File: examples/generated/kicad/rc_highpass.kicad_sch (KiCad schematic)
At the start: 3 parts

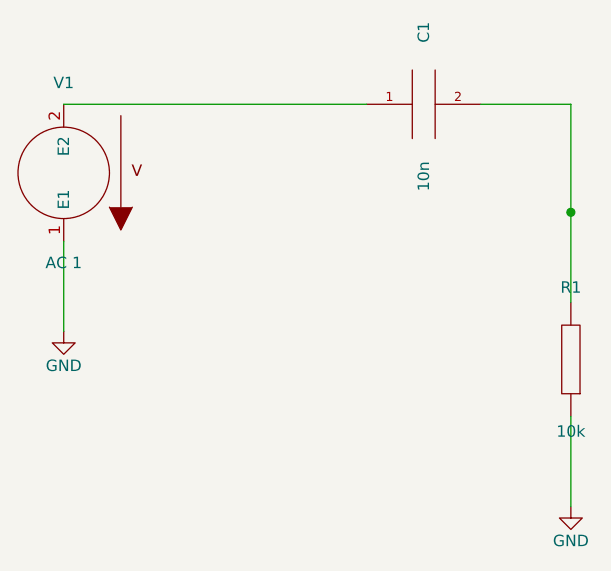
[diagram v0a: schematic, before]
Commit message: Attempt to fix more terminal issues.
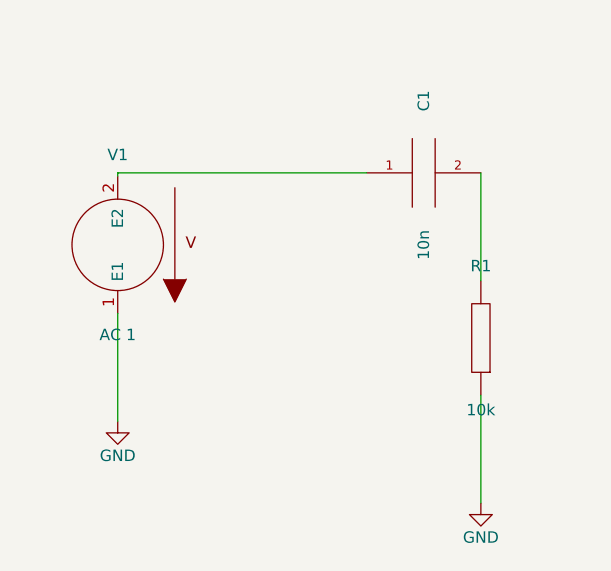
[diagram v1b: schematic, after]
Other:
- moved on the sheet: C1, R1, V1
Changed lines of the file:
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@@
     (comment 1 "Generated by mixedsig2cad")
   )
-  (symbol (lib_id "VSOURCE") (at 50.00 78.00 180) (unit 1)
+  (symbol (lib_id "VSOURCE") (at 56.00 86.00 180) (unit 1)
     (in_bom yes) (on_board yes)
-    (property "Reference" "V1" (at 50.0 68.0 0)
+    (property "Reference" "V1" (at 56.0 76.0 0)
       (effects (font (size 1.27 1.27)))
     )
-    (property "Value" "AC 1" (at 50.0 88.0 0)
+    (property "Value" "AC 1" (at 56.0 96.0 0)
       (effects (font (size 1.27 1.27)))
     )
@@
     )
   )
-  (symbol (lib_id "CAP") (at 90.00 70.38 90) (unit 1)
+  (symbol (lib_id "GND") (at 56.00 105.62 0) (unit 1)
     (in_bom yes) (on_board yes)
-    (property "Reference" "C1" (at 90.0 62.379999999999995 0)
-      (effects (font (size 1.27 1.27)))
+    (property "Reference" "#PWR0001" (at 56.0 101.81 0)
+      (effects (font (size 1.27 1.27)) hide)
     )
-    (property "Value" "10n" (at 90.0 78.38 0)
+    (property "Value" "GND" (at 56.0 109.43 0)
       (effects (font (size 1.27 1.27)))
     )
@@
     )
   )
-  (symbol (lib_id "R") (at 106.35 98.73 180) (unit 1)
+  (symbol (lib_id "CAP") (at 90.00 78.00 90) (unit 1)
     (in_bom yes) (on_board yes)
-    (property "Reference" "R1" (at 106.35 90.73 0)
+    (property "Reference" "C1" (at 90.0 70.0 0)
       (effects (font (size 1.27 1.27)))
     )
-    (property "Value" "10k" (at 106.35 106.73 0)
+    (property "Value" "10n" (at 90.0 86.0 0)
       (effects (font (size 1.27 1.27)))
     )
@@
     )
   )
-  (symbol (lib_id "GND") (at 50.00 95.62 0) (unit 1)
+  (symbol (lib_id "R") (at 96.35 96.35 180) (unit 1)
     (in_bom yes) (on_board yes)
-    (property "Reference" "#PWR0001" (at 50.0 91.81 0)
-      (effects (font (size 1.27 1.27)) hide)
+    (property "Reference" "R1" (at 96.35 88.35 0)
+      (effects (font (size 1.27 1.27)))
     )
-    (property "Value" "GND" (at 50.0 99.43 0)
+    (property "Value" "10k" (at 96.35 104.35 0)
       (effects (font (size 1.27 1.27)))
     )
@@
     )
   )
-  (symbol (lib_id "GND") (at 106.35 115.08 0) (unit 1)
+  (symbol (lib_id "GND") (at 96.35 114.70 0) (unit 1)
     (in_bom yes) (on_board yes)
-    (property "Reference" "#PWR0002" (at 106.35 111.27 0)
+    (property "Reference" "#PWR0002" (at 96.35 110.89 0)
       (effects (font (size 1.27 1.27)) hide)
     )
-    (property "Value" "GND" (at 106.35 118.89 0)
+    (property "Value" "GND" (at 96.35 118.51 0)
       (effects (font (size 1.27 1.27)))
     )
@@
     )
   )
-  (wire (pts (xy 50.00 70.38) (xy 83.65 70.38))
+  (wire (pts (xy 96.35 102.70) (xy 96.35 114.70))
     (stroke (width 0) (type solid) (color 0 0 0 0))
   )
-  (wire (pts (xy 96.35 70.38) (xy 106.35 70.38))
+  (wire (pts (xy 56.00 93.62) (xy 56.00 105.62))
     (stroke (width 0) (type solid) (color 0 0 0 0))
   )
-  (wire (pts (xy 106.35 70.38) (xy 106.35 82.38))
+  (wire (pts (xy 56.00 78.38) (xy 56.00 78.00))
     (stroke (width 0) (type solid) (color 0 0 0 0))
   )
-  (wire (pts (xy 106.35 92.38) (xy 106.35 82.38))
+  (wire (pts (xy 56.00 78.00) (xy 83.65 78.00))
     (stroke (width 0) (type solid) (color 0 0 0 0))
   )
-  (wire (pts (xy 50.00 85.62) (xy 50.00 95.62))
+  (wire (pts (xy 96.35 78.00) (xy 96.35 90.00))
     (stroke (width 0) (type solid) (color 0 0 0 0))
   )
-  (wire (pts (xy 106.35 105.08) (xy 106.35 115.08))
-    (stroke (width 0) (type solid) (color 0 0 0 0))
-  )
-  (junction (at 106.35 82.38) (diameter 1.016) (color 0 0 0 0))
   (sheet_instances
     (path "/" (page "1"))
@@
   (symbol_instances
     (path "/236c4ed6-19b0-5092-bdb2-caacc762cc72" (reference "V1") (unit 1) (value "AC 1") (footprint ""))
+    (path "/d76d2626-14f8-5e35-8eaa-916a5b195b2f" (reference "#PWR0001") (unit 1) (value "GND") (footprint ""))
     (path "/58c843b2-6559-5058-b688-d947388eea66" (reference "C1") (unit 1) (value "10n") (footprint ""))
     (path "/ded07918-9cee-5a7e-a275-1ccd4f0b81cb" (reference "R1") (unit 1) (value "10k") (footprint ""))
-    (path "/d76d2626-14f8-5e35-8eaa-916a5b195b2f" (reference "#PWR0001") (unit 1) (value "GND") (footprint ""))
     (path "/866988e1-0e40-5667-846e-d709fa13875c" (reference "#PWR0002") (unit 1) (value "GND") (footprint ""))
   )
